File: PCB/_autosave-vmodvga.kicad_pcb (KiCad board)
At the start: 2 copper layers, 80 x 60.1 mm, 70 parts, among them J1 DE-15, J2 DE-15, J3 VHDCI, P1 50R, P2 50R, P3 50R, P4 50R, P5 CONN_1, P6 CONN_1, U1 ADP3303-3V3, U2 ADP3334, U3 AD9984, U4 ADP3334

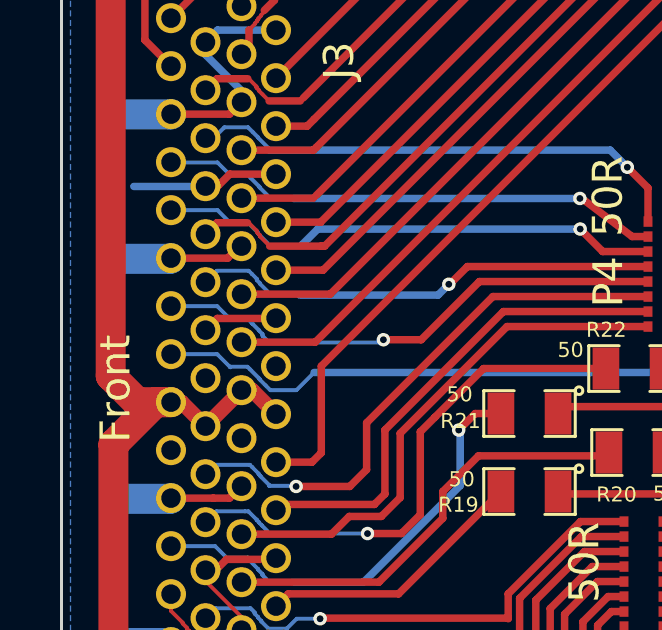
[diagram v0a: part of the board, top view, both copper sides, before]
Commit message: PCB Routing
70% tracks routed. Fine tuning remaining
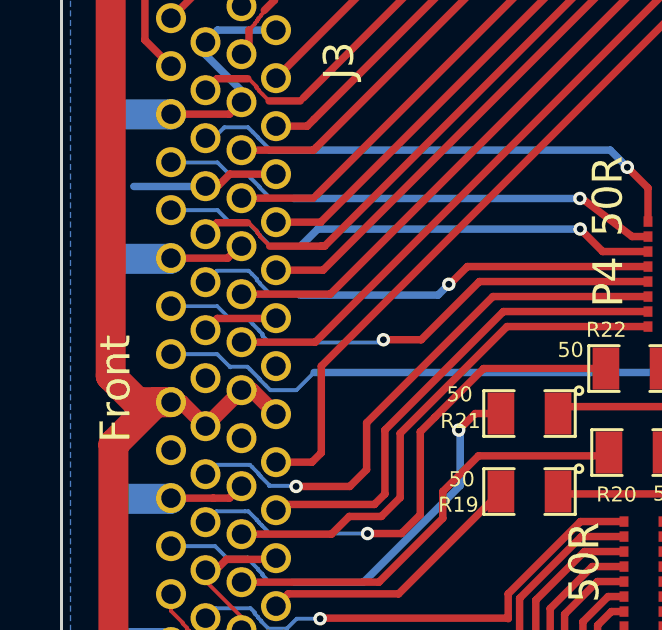
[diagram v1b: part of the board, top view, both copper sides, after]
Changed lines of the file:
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@@
     (links 253)
     (no_connects 2)
-    (area 46.3975 49.249999 167.950001 168.4525)
+    (area 87.849999 49.249999 209.9023 109.450001)
     (thickness 1.6)
     (drawings 7)
@@
   (gr_line (start 167.9 109.35) (end 167.9 49.35) (angle 90) (layer Edge.Cuts) (width 0.1))
   (target plus (at 87.9 109.25) (size 0.005) (width 0.1) (layer Edge.Cuts))
-  (target plus (at 46.4 168.45) (size 0.005) (width 0.1) (layer Edge.Cuts))
+  (target plus (at 209.8998 79.4484) (size 0.005) (width 0.1) (layer Edge.Cuts))
   (segment (start 106.65 87.2) (end 106.65 89.24) (width 0.25) (layer F.Cu) (net 1))
   (segment (start 104.57 91.32) (end 95.05 91.32) (width 0.25) (layer F.Cu) (net 1) (status 20))
@@
   (segment (start 93.01 81.81) (end 92.7 82.12) (width 0.13) (layer B.Cu) (net 18) (status 30))
   (segment (start 94.18 81.81) (end 93.01 81.81) (width 0.13) (layer B.Cu) (net 18) (status 20))
-  (segment (start 94.27 77.11) (end 94.09 76.93) (width 0.13) (layer B.Cu) (net 19))
-  (segment (start 93.09 76.52) (end 91.55 76.52) (width 0.13) (layer B.Cu) (net 19) (status 20))
-  (segment (start 93.5 76.93) (end 93.09 76.52) (width 0.13) (layer B.Cu) (net 19))
-  (segment (start 94.09 76.93) (end 93.5 76.93) (width 0.13) (layer B.Cu) (net 19))
+  (segment (start 94.27 77.11) (end 94.09 76.93) (width 0.125) (layer B.Cu) (net 19))
+  (segment (start 94.09 76.93) (end 93.5 76.93) (width 0.125) (layer B.Cu) (net 19))
+  (segment (start 93.5 76.93) (end 93.09 76.52) (width 0.125) (layer B.Cu) (net 19))
+  (segment (start 93.09 76.52) (end 91.55 76.52) (width 0.125) (layer B.Cu) (net 19) (status 20))
   (segment (start 94.48 77.33) (end 94.48 77.32) (width 0.13) (layer B.Cu) (net 19))
   (segment (start 94.6 77.51) (end 94.6 77.45) (width 0.13) (layer B.Cu) (net 19))
